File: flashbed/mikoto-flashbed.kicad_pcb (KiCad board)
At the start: 2 copper layers, 46 x 46 mm, 10 parts, among them J1 Conn_01x01, J2 Conn_01x01, J3 Conn_01x01, J4 Conn_01x01, J7 Conn_01x05, J8 Conn_01x01, SW1 TVBP06, U1 mikoto-pins

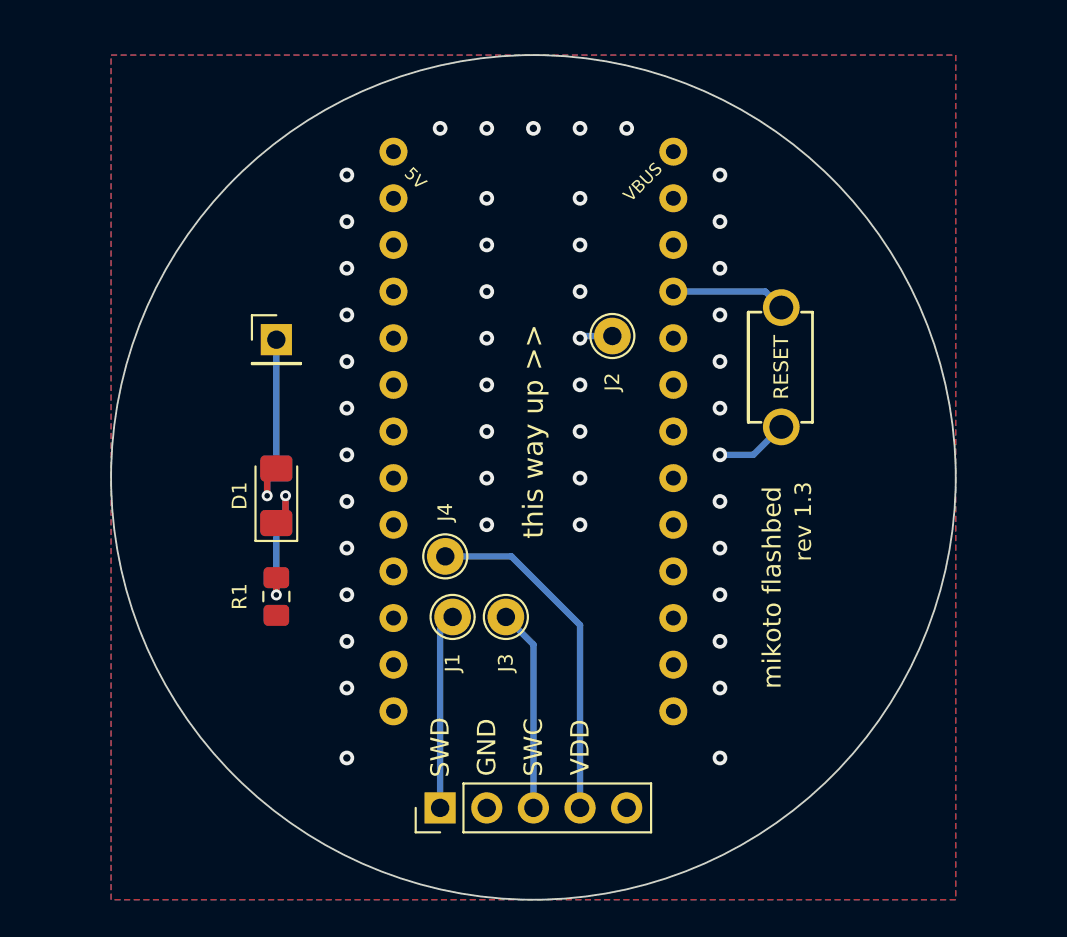
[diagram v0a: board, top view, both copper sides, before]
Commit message: update flashbed
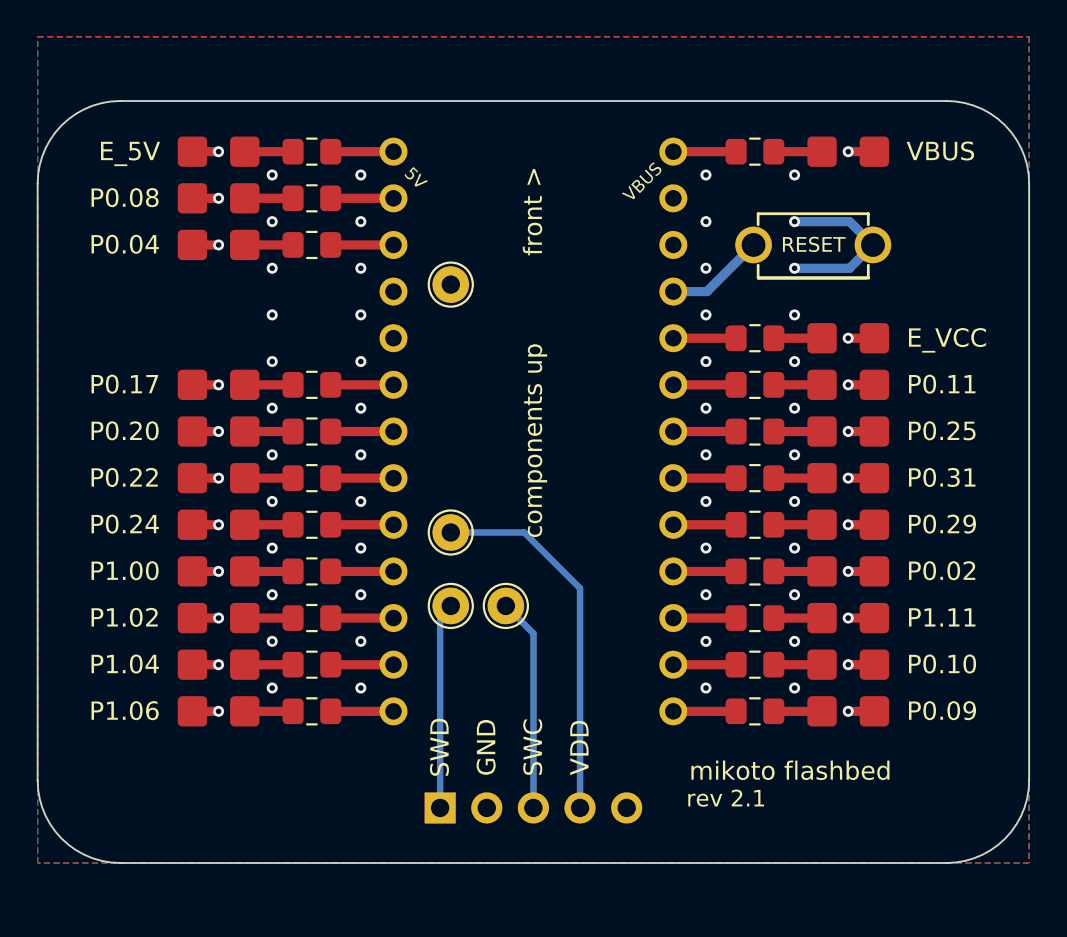
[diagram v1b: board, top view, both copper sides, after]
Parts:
- removed J8: Conn_01x01, Connector_PinHeader_2.54mm:PinHeader_1x01_P2.54mm_Vertical
- added D10: LED_Small, footprints:LED_1206_3216M_Castellated-nosilk, F.Cu at (-17.1, 12.7)
- added D11: LED_Small, footprints:LED_1206_3216M_Castellated-nosilk, F.Cu at (-17.1, 15.2)
- added D12: LED_Small, footprints:LED_1206_3216M_Castellated-nosilk, F.Cu at (17.1, 15.2)
- added D13: LED_Small, footprints:LED_1206_3216M_Castellated-nosilk, F.Cu at (17.1, 12.7)
- added D14: LED_Small, footprints:LED_1206_3216M_Castellated-nosilk, F.Cu at (17.1, 10.2)
- added D15: LED_Small, footprints:LED_1206_3216M_Castellated-nosilk, F.Cu at (17.1, 7.62)
- added D16: LED_Small, footprints:LED_1206_3216M_Castellated-nosilk, F.Cu at (17.1, 5.08)
- added D17: LED_Small, footprints:LED_1206_3216M_Castellated-nosilk, F.Cu at (17.1, 2.54)
- added D18: LED_Small, footprints:LED_1206_3216M_Castellated-nosilk, F.Cu at (17.1, 0.00)
- added D19: LED_Small, footprints:LED_1206_3216M_Castellated-nosilk, F.Cu at (17.1, -2.54)
- added D2: LED_Small, footprints:LED_1206_3216M_Castellated-nosilk, F.Cu at (-17.1, -12.7)
- added D20: LED_Small, footprints:LED_1206_3216M_Castellated-nosilk, F.Cu at (17.1, -5.08)
- added D21: LED_Small, footprints:LED_1206_3216M_Castellated-nosilk, F.Cu at (17.1, -15.2)
- added D3: LED_Small, footprints:LED_1206_3216M_Castellated-nosilk, F.Cu at (-17.1, -10.2)
- added D4: LED_Small, footprints:LED_1206_3216M_Castellated-nosilk, F.Cu at (-17.1, -2.54)
- added D5: LED_Small, footprints:LED_1206_3216M_Castellated-nosilk, F.Cu at (-17.1, 0.00)
- added D6: LED_Small, footprints:LED_1206_3216M_Castellated-nosilk, F.Cu at (-17.1, 2.54)
- added D7: LED_Small, footprints:LED_1206_3216M_Castellated-nosilk, F.Cu at (-17.1, 5.08)
- added D8: LED_Small, footprints:LED_1206_3216M_Castellated-nosilk, F.Cu at (-17.1, 7.62)
- added D9: LED_Small, footprints:LED_1206_3216M_Castellated-nosilk, F.Cu at (-17.1, 10.2)
- added R10: 2.2k, Resistor_SMD:R_0805_2012Metric_Pad1.15x1.40mm_HandSolder, F.Cu at (-12.1, 12.7)
- added R11: 2.2k, Resistor_SMD:R_0805_2012Metric_Pad1.15x1.40mm_HandSolder, F.Cu at (-12.1, 15.2)
- added R12: 2.2k, Resistor_SMD:R_0805_2012Metric_Pad1.15x1.40mm_HandSolder, F.Cu at (12.1, 15.2)
- added R13: 2.2k, Resistor_SMD:R_0805_2012Metric_Pad1.15x1.40mm_HandSolder, F.Cu at (12.1, 12.7)
- added R14: 2.2k, Resistor_SMD:R_0805_2012Metric_Pad1.15x1.40mm_HandSolder, F.Cu at (12.1, 10.2)
- added R15: 2.2k, Resistor_SMD:R_0805_2012Metric_Pad1.15x1.40mm_HandSolder, F.Cu at (12.1, 7.62)
- added R16: 2.2k, Resistor_SMD:R_0805_2012Metric_Pad1.15x1.40mm_HandSolder, F.Cu at (12.1, 5.08)
- added R17: 2.2k, Resistor_SMD:R_0805_2012Metric_Pad1.15x1.40mm_HandSolder, F.Cu at (12.1, 2.54)
- added R18: 2.2k, Resistor_SMD:R_0805_2012Metric_Pad1.15x1.40mm_HandSolder, F.Cu at (12.1, 0.00)
- added R19: 2.2k, Resistor_SMD:R_0805_2012Metric_Pad1.15x1.40mm_HandSolder, F.Cu at (12.1, -2.54)
- added R2: 2.2k, Resistor_SMD:R_0805_2012Metric_Pad1.15x1.40mm_HandSolder, F.Cu at (-12.1, -12.7)
- added R20: 2.2k, Resistor_SMD:R_0805_2012Metric_Pad1.15x1.40mm_HandSolder, F.Cu at (12.1, -5.08)
- added R21: 2.2k, Resistor_SMD:R_0805_2012Metric_Pad1.15x1.40mm_HandSolder, F.Cu at (12.1, -15.2)
- added R3: 2.2k, Resistor_SMD:R_0805_2012Metric_Pad1.15x1.40mm_HandSolder, F.Cu at (-12.1, -10.2)
- added R4: 2.2k, Resistor_SMD:R_0805_2012Metric_Pad1.15x1.40mm_HandSolder, F.Cu at (-12.1, -2.54)
- added R5: 2.2k, Resistor_SMD:R_0805_2012Metric_Pad1.15x1.40mm_HandSolder, F.Cu at (-12.1, 0.00)
- added R6: 2.2k, Resistor_SMD:R_0805_2012Metric_Pad1.15x1.40mm_HandSolder, F.Cu at (-12.1, 2.54)
- added R7: 2.2k, Resistor_SMD:R_0805_2012Metric_Pad1.15x1.40mm_HandSolder, F.Cu at (-12.1, 5.08)
- added R8: 2.2k, Resistor_SMD:R_0805_2012Metric_Pad1.15x1.40mm_HandSolder, F.Cu at (-12.1, 7.62)
- added R9: 2.2k, Resistor_SMD:R_0805_2012Metric_Pad1.15x1.40mm_HandSolder, F.Cu at (-12.1, 10.2)
- D1: footprint LED_SMD:LED_1206_3216Metric_Pad1.42x1.75mm_HandSolder -> footprints:LED_1206_3216M_Castellated-nosilk
- U1: footprint footprints:mikoto-pins -> footprints:mikoto-pins-bigger-holes
- moved R1 24.3 mm to (-12.1, -15.2), turned to 180 degrees
- moved D1 19.0 mm to (-17.1, -15.2), turned to 0 degrees
- moved J2 9.23 mm to (-4.50, -8.00)
- moved SW1 6.88 mm to (15.2, -10.2), turned to 0 degrees
- moved J4 1.33 mm to (-4.50, 5.50)
- moved J1 0.61 mm to (-4.50, 9.50)
- moved J3 0.60 mm to (-1.50, 9.50)
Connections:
- D1 pad 1: Net-(D1-Pad1) -> GND
- R1 pad 1: Net-(D1-Pad1) -> EXT_5V
- R1 pad 2: GND -> Net-(D1-Pad2)
- U1 pad 1: unconnected-(U1-Pad1) -> EXT_5V
- U1 pad 10: unconnected-(U1-Pad10) -> P1.00
- U1 pad 11: unconnected-(U1-Pad11) -> P1.02
- U1 pad 12: unconnected-(U1-Pad12) -> P1.04
- U1 pad 13: unconnected-(U1-Pad13) -> P1.06
- U1 pad 14: unconnected-(U1-Pad14) -> P0.09
- U1 pad 15: unconnected-(U1-Pad15) -> P0.10
- U1 pad 16: unconnected-(U1-Pad16) -> P1.11
- U1 pad 17: unconnected-(U1-Pad17) -> P0.02
- U1 pad 18: unconnected-(U1-Pad18) -> P0.29
- U1 pad 19: unconnected-(U1-Pad19) -> P0.31
- U1 pad 2: unconnected-(U1-Pad2) -> P0.08
- U1 pad 20: unconnected-(U1-Pad20) -> P0.25
- U1 pad 21: unconnected-(U1-Pad21) -> P0.11
- U1 pad 22: unconnected-(U1-Pad22) -> EXT_VCC
- U1 pad 25: unconnected-(U1-Pad25) -> VBAT
- U1 pad 26: unconnected-(U1-Pad26) -> VBUS
- U1 pad 3: unconnected-(U1-Pad3) -> P0.04
- U1 pad 6: unconnected-(U1-Pad6) -> P0.17
- U1 pad 7: unconnected-(U1-Pad7) -> P0.20
- U1 pad 8: unconnected-(U1-Pad8) -> P0.22
- U1 pad 9: unconnected-(U1-Pad9) -> P0.24
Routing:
- net GND: track 5.78 -> 40.8 mm, vias 47 -> 69
- net Net-(D1-Pad1): track 8.24 -> 0.00 mm, vias 2 -> 0
- net Net-(D1-Pad2): track 10.4 -> 2.57 mm, vias 1 -> 0
- net VBUS: track 0.00 -> 3.42 mm
- net P1.11: track 0.00 -> 3.42 mm
- net P1.06: track 0.00 -> 3.42 mm
- net P1.04: track 0.00 -> 3.42 mm
- net P1.02: track 0.00 -> 3.42 mm
- net P1.00: track 0.00 -> 3.42 mm
- net P0.31: track 0.00 -> 3.42 mm
- net P0.29: track 0.00 -> 3.42 mm
- net P0.25: track 0.00 -> 3.42 mm
- net P0.24: track 0.00 -> 3.42 mm
- net P0.22: track 0.00 -> 3.42 mm
- net P0.20: track 0.00 -> 3.42 mm
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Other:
- board size 46 x 46 mm -> 54 x 41.5 mm
- board text added: "E_5V"
- board text added: "E_VCC"
- board text added: "P0.02"
- board text added: "P0.04"
- board text added: "P0.08"
- board text added: "P0.09"
- board text added: "P0.10"
- board text added: "P0.11"
- board text added: "P0.17"
- board text added: "P0.20"
- board text added: "P0.22"
- board text added: "P0.24"
- board text added: "P0.25"
- board text added: "P0.29"
- board text added: "P0.31"
- board text added: "P1.00"
- board text added: "P1.02"
- board text added: "P1.04"
- board text added: "P1.06"
- board text added: "P1.11"
- board text added: "VBUS"
- board text added: "components up"
- board text added: "front >"
- board text added: "rev 2.1"
- board text removed: "rev 1.3"
- board text removed: "this way up >>"
